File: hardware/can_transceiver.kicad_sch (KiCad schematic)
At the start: 10 parts

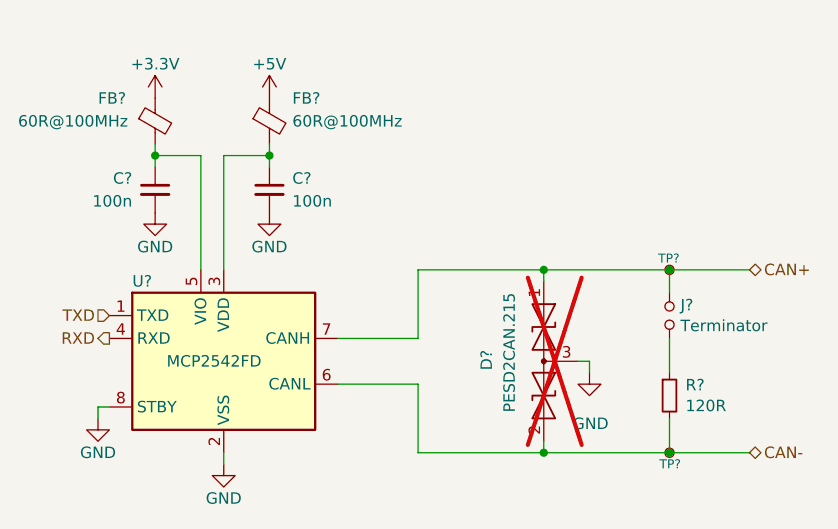
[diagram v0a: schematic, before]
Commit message: Add the Cube project
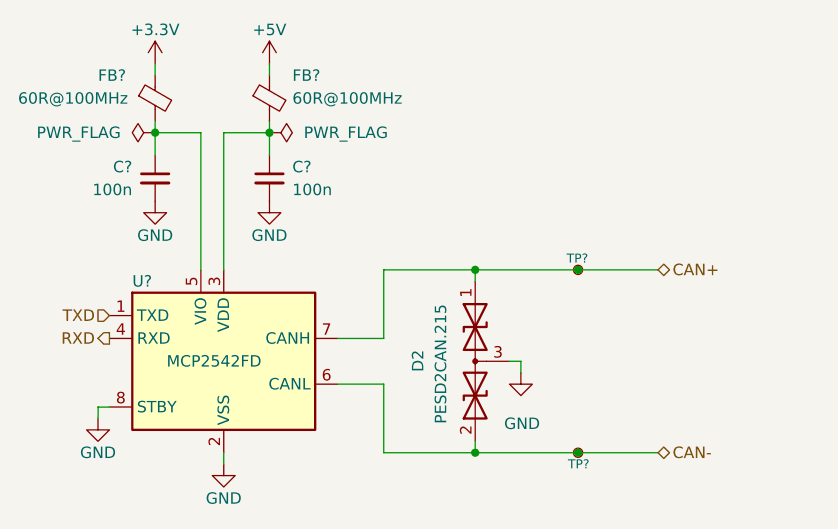
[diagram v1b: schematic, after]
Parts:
- removed D?: PESD2CAN.215, Package_TO_SOT_SMD:SOT-23, symbol Local_Library:D_TVS_x2_AAC-Device
- removed J?: Terminator, Connector_PinHeader_2.54mm:PinHeader_1x02_P2.54mm_Vertical, symbol Local_Library:Jumper_NO_Small-Device
- removed R?: 120R, Resistor_SMD:R_0402_1005Metric, symbol Device:R_Small
- added D2: PESD2CAN.215, Package_TO_SOT_SMD:SOT-23, symbol Device:D_TVS_Dual_AAC
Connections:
- net CAN+: now also D2.1 (A1)
- net CAN-: now also D2.2 (A2)
- net GND: now also D2.3 (common)
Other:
- moved on the sheet: C?, FB?, TP?
